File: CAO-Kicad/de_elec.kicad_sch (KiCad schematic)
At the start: 17 parts, among them J1 ICSP, SW1 COMMUTATEUR VIBRATION, U1 puce de microcontrôleur IC AT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

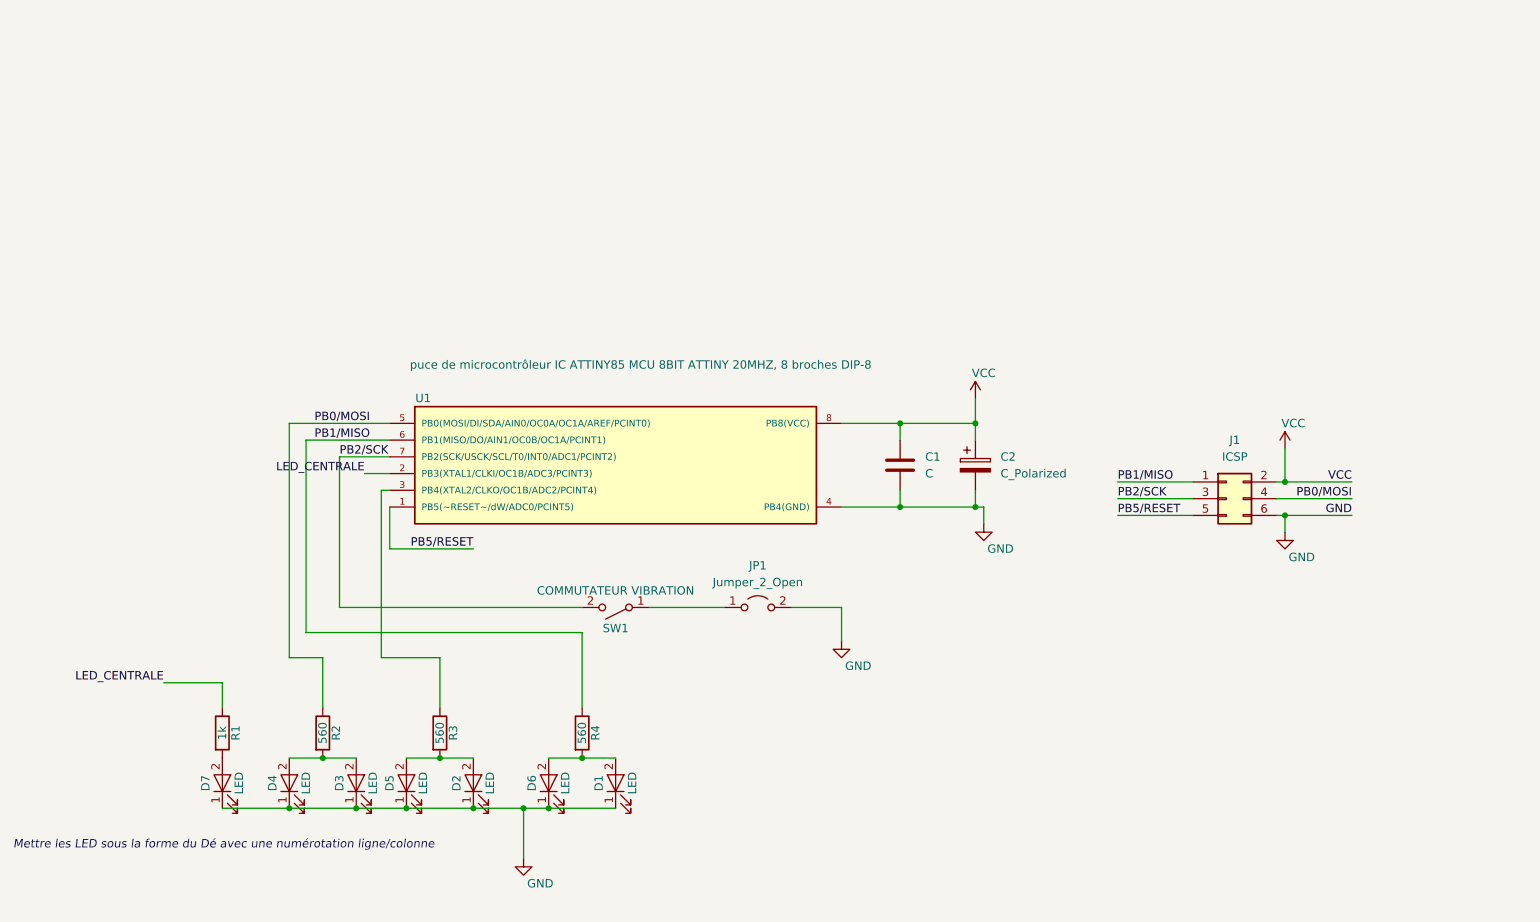
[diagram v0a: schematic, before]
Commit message: Ajout des docs et images
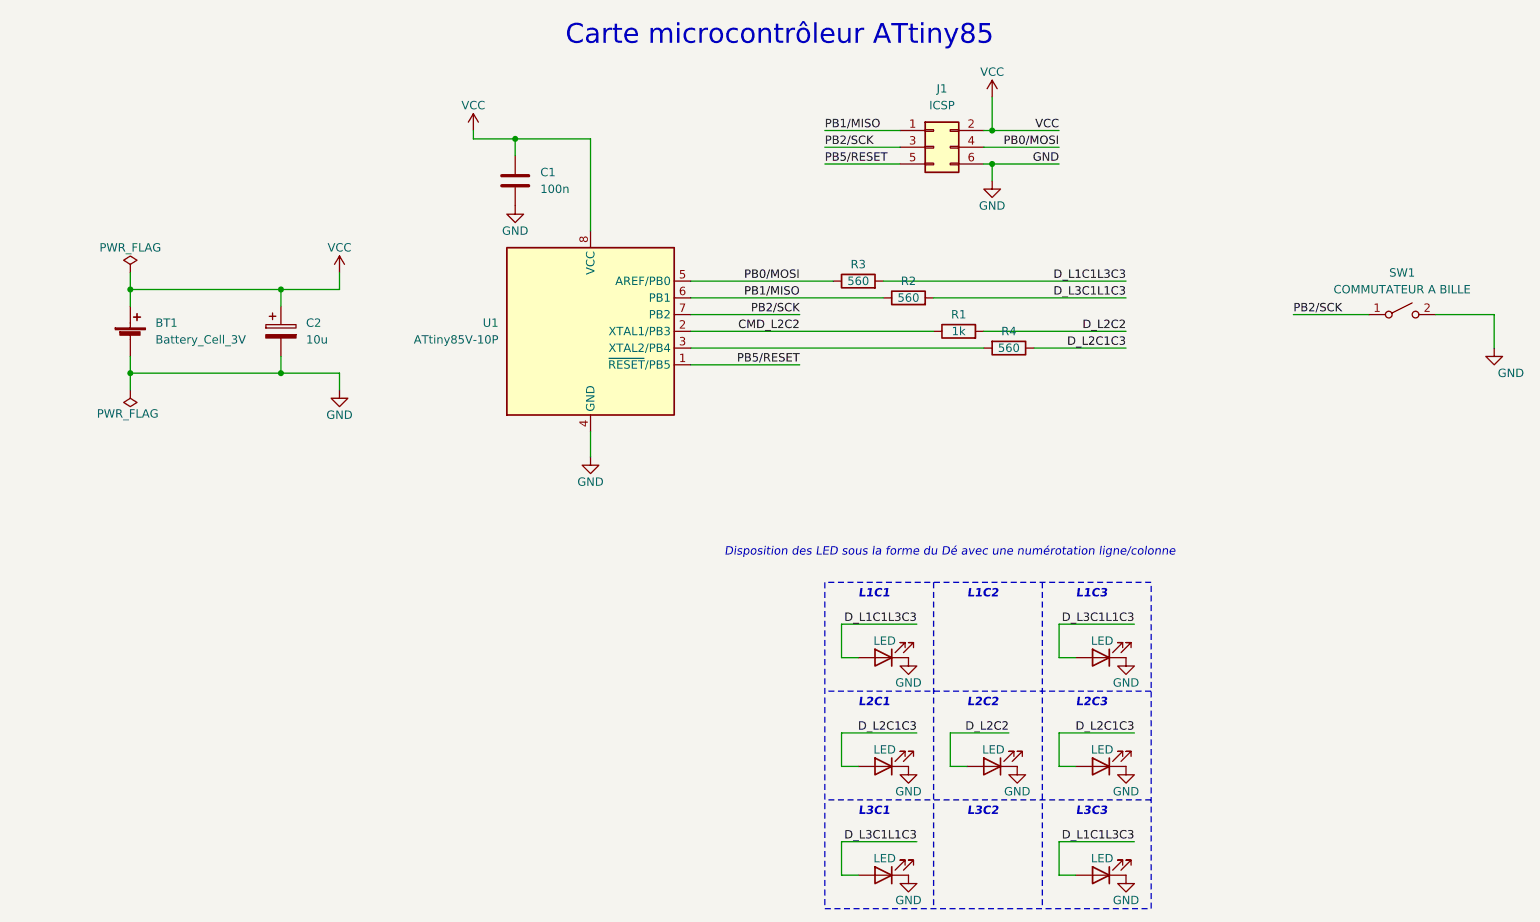
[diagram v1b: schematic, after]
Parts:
- removed D1, D2, D3, D4, D5, D6, D7: LED, LEDs:LED_D5.0mm, symbol kicad_dÚ-rescue:LED
- removed JP1: Jumper_2_Open, symbol Jumper:Jumper_2_Open
- removed R1: 1k, Resistors_SMD:R_0805_HandSoldering, symbol kicad_dÚ-rescue:R
- removed R2, R3, R4: 560, Resistors_SMD:R_0805_HandSoldering, symbol kicad_dÚ-rescue:R
- removed SW1: COMMUTATEUR VIBRATION, Capacitors_THT:CP_Radial_D5.0mm_P2.50mm, symbol kicad_dÚ-rescue:SW_SPST
- removed U1: puce de microcontrôleur IC ATTINY85 MCU 8BIT ATTI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, Housings_DIP:DIP-8_W7.62mm, symbol kicad_dÚ-rescue:ATTINY85-20PU
- added BT1: Battery_Cell_3V, symbol Device:Battery_Cell
- added D_L1C1, D_L1C3, D_L2C1, D_L2C2, D_L2C3, D_L3C1, D_L3C3: LED, symbol Device:LED
- added R1: 1k, symbol Device:R
- added R2, R3, R4: 560, symbol Device:R
- added SW1: COMMUTATEUR A BILLE, Capacitors_THT:CP_Radial_D5.0mm_P2.50mm, symbol Switch:SW_SPST
- added U1: ATtiny85V-10P, Package_DIP:DIP-8_W7.62mm, symbol MCU_Microchip_ATtiny:ATtiny85V-10P
- C1: value C -> 100n
- C2: value C_Polarized -> 10u
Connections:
- net GND: now also BT1.2 (-), D_L1C1.1 (K), D_L1C3.1 (K), D_L2C1.1 (K), D_L2C2.1 (K), D_L2C3.1 (K), D_L3C1.1 (K), D_L3C3.1 (K), SW1.2 (B), U1.4 (GND)
- net PB0/MOSI: now also R3.1, U1.5 (AREF/PB0)
- net PB1/MISO: now also R2.1, U1.6 (PB1)
- net PB2/SCK: now also SW1.1 (A), U1.7 (PB2)
- net PB5/RESET: now also U1.1 (~{RESET}/PB5)
- net VCC: now also BT1.1 (+), U1.8 (VCC)
- new net: R4.2, U1.3 (XTAL2/PB4)
- new net CMD_L2C2: R1.1, U1.2 (XTAL1/PB3)
- new net D_L1C1L3C3: D_L1C1.2 (A), D_L3C3.2 (A), R3.2
- new net D_L2C1C3: D_L2C1.2 (A), D_L2C3.2 (A), R4.1
- new net D_L2C2: D_L2C2.2 (A), R1.2
- new net D_L3C1L1C3: D_L1C3.2 (A), D_L3C1.2 (A), R2.2
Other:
- note added: "Carte microcontrôleur ATtiny85"
- note added: "Disposition des LED sous la forme du Dé avec une numérotation ligne/colonne"
- note added: "L1C1"
- note added: "L1C2"
- note added: "L1C3"
- note added: "L2C1"
- note added: "L2C2"
- note added: "L2C3"
- note added: "L3C1"
- note added: "L3C2"
- note added: "L3C3"
- note removed: "Mettre les LED sous la forme du Dé avec une numérotation ligne/colonne"
- moved on the sheet: C1, C2, J1
